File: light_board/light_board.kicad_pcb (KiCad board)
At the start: 2 copper layers, 31.8 x 38.1 mm, 16 parts, among them J1 CONN_01X02, J2 Led_Connector, J3 Power_Connector, Q1 FDC658AP, U1 LM3409MY

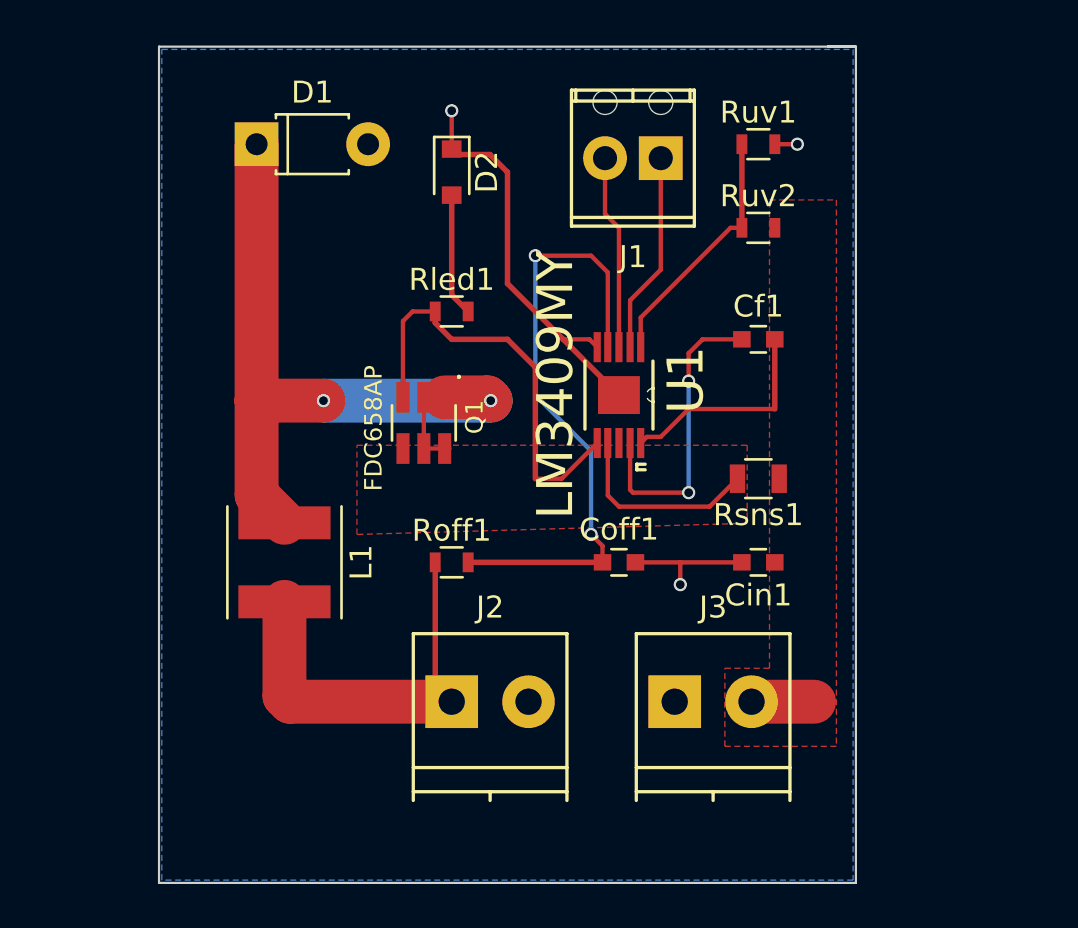
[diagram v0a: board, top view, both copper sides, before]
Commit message: final modifications
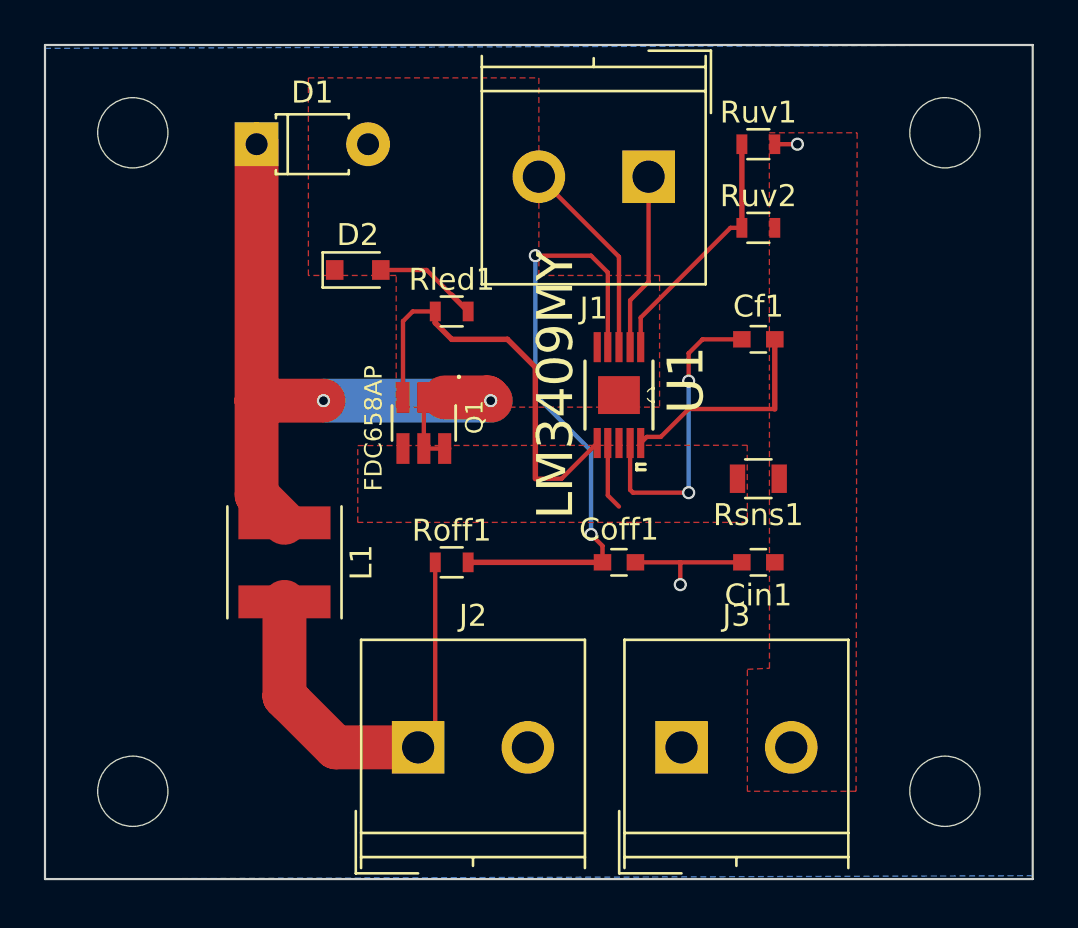
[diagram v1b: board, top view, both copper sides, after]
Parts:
- added ?: , Mounting_Holes:MountingHole_3.2mm_M3, F.Cu at (162.0, 126.0)
- added ?: , Mounting_Holes:MountingHole_3.2mm_M3, F.Cu at (162.0, 96.0)
- added ?: , Mounting_Holes:MountingHole_3.2mm_M3, F.Cu at (199.0, 126.0)
- added ?: , Mounting_Holes:MountingHole_3.2mm_M3, F.Cu at (199.0, 96.0)
- D2: value LED -> Gate
- J1: value CONN_01X02 -> PWM; footprint Connectors_Terminal_Blocks:TerminalBlock_Pheonix_MPT-2.54mm_2pol -> Connectors_Terminal_Blocks:TerminalBlock_Philmore_TB132_02x5mm_Straight
- J2: value Led_Connector -> Led; footprint Connectors_Terminal_Blocks:TerminalBlock_Pheonix_PT-3.5mm_2pol -> Connectors_Terminal_Blocks:TerminalBlock_Philmore_TB132_02x5mm_Straight
- J3: value Power_Connector -> Power; footprint Connectors_Terminal_Blocks:TerminalBlock_Pheonix_PT-3.5mm_2pol -> Connectors_Terminal_Blocks:TerminalBlock_Philmore_TB132_02x5mm_Straight
- moved D2 6.18 mm to (172.2, 102.2), turned to 0 degrees
- moved J2 2.58 mm to (175.0, 124.0)
- moved J3 2.10 mm to (187.0, 124.0)
- moved J1 1.01 mm to (185.5, 98.0)
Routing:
- net GND: track 25.5 -> 6.89 mm, vias 3 -> 2
- net /CSN: track 9.03 -> 3.11 mm
- net /CSP: track 13.7 -> 10.8 mm
- net /LEDVcc: track 18.7 -> 20.5 mm
- net Net-(D2-Pad2): track 5.86 -> 4.76 mm
- net /notUsed: track 9.19 -> 8.11 mm
- added copper zone on F.Cu, net GND
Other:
- board size 31.8 x 38.1 mm -> 45 x 38 mm
